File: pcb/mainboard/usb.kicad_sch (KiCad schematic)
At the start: 35 parts, among them J601 USB_A, J602 USB_A, J603 USB_C_Receptacle_USB2.0, J604 USB_B_Micro, U601 USB2514B_Bi, U602 AP2171W, U603 AP2171W, U604 FUSB302BMPX, U605 USBLC6-2P6, Y601 24MHz

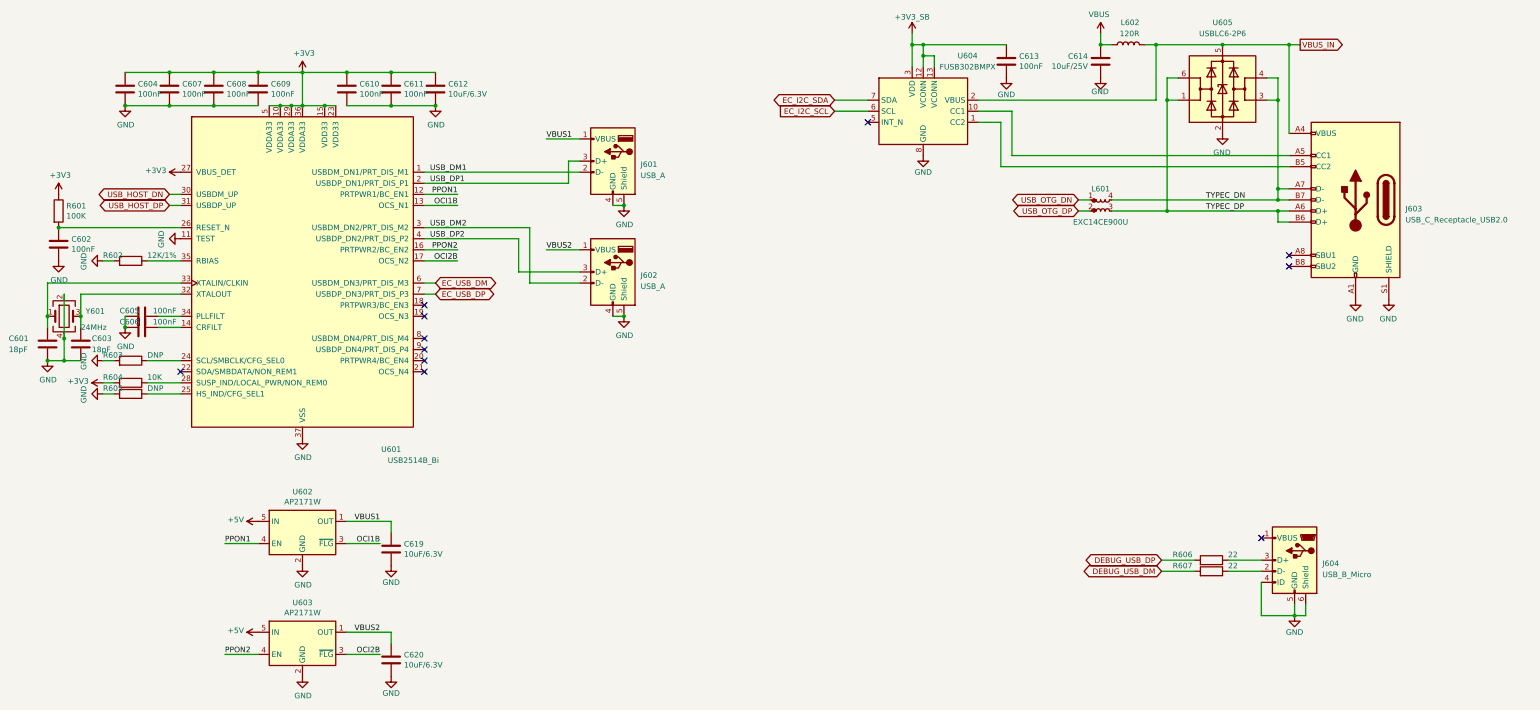
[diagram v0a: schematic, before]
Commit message: - pcb: finishing layout r0p1
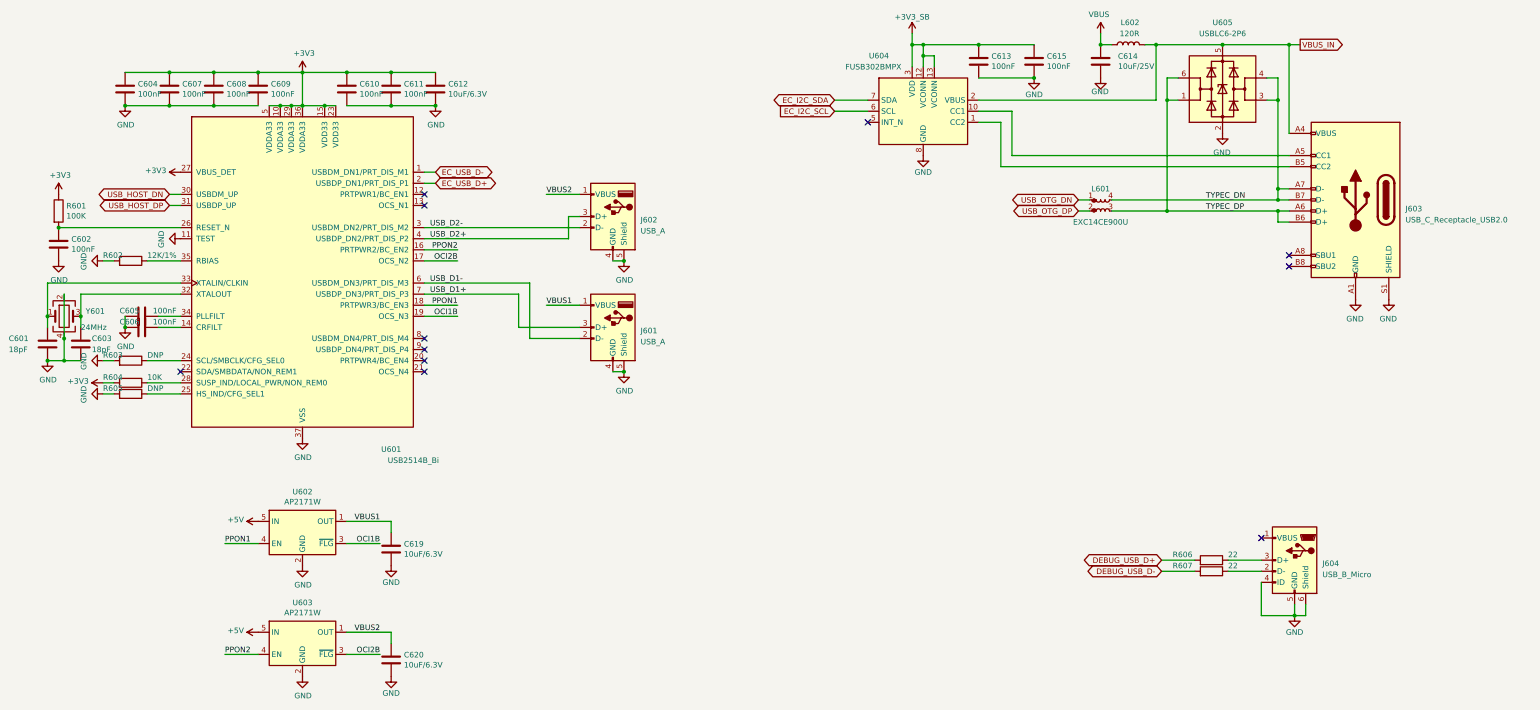
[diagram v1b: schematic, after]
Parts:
- added C615: 100nF, Capacitor_SMD:C_0402_1005Metric, symbol Device:C
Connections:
- net +3V3_SB: now also C615.1
- net GND: now also C615.2
- net OCI1B: now also U601.19 (OCS_N3); no longer U601.13 (OCS_N1)
- net PPON1: now also U601.18 (PRTPWR3/BC_EN3); no longer U601.12 (PRTPWR1/BC_EN1)
- net DEBUG_USB_DM renamed DEBUG_USB_D-
- net DEBUG_USB_DP renamed DEBUG_USB_D+
- net EC_USB_DM renamed USB_D1-
- net USB_D1-: now also J601.2 (D-)
- net EC_USB_DP renamed USB_D1+
- net USB_D1+: now also J601.3 (D+)
- net USB_DM1 renamed EC_USB_D-
- net EC_USB_D-: no longer J601.2 (D-)
- net USB_DM2 renamed USB_D2-
- net USB_DP1 renamed EC_USB_D+
- net EC_USB_D+: no longer J601.3 (D+)
- net USB_DP2 renamed USB_D2+
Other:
- moved on the sheet: C613, J601, J602
